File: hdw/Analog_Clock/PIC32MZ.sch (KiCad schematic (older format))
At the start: 3 parts

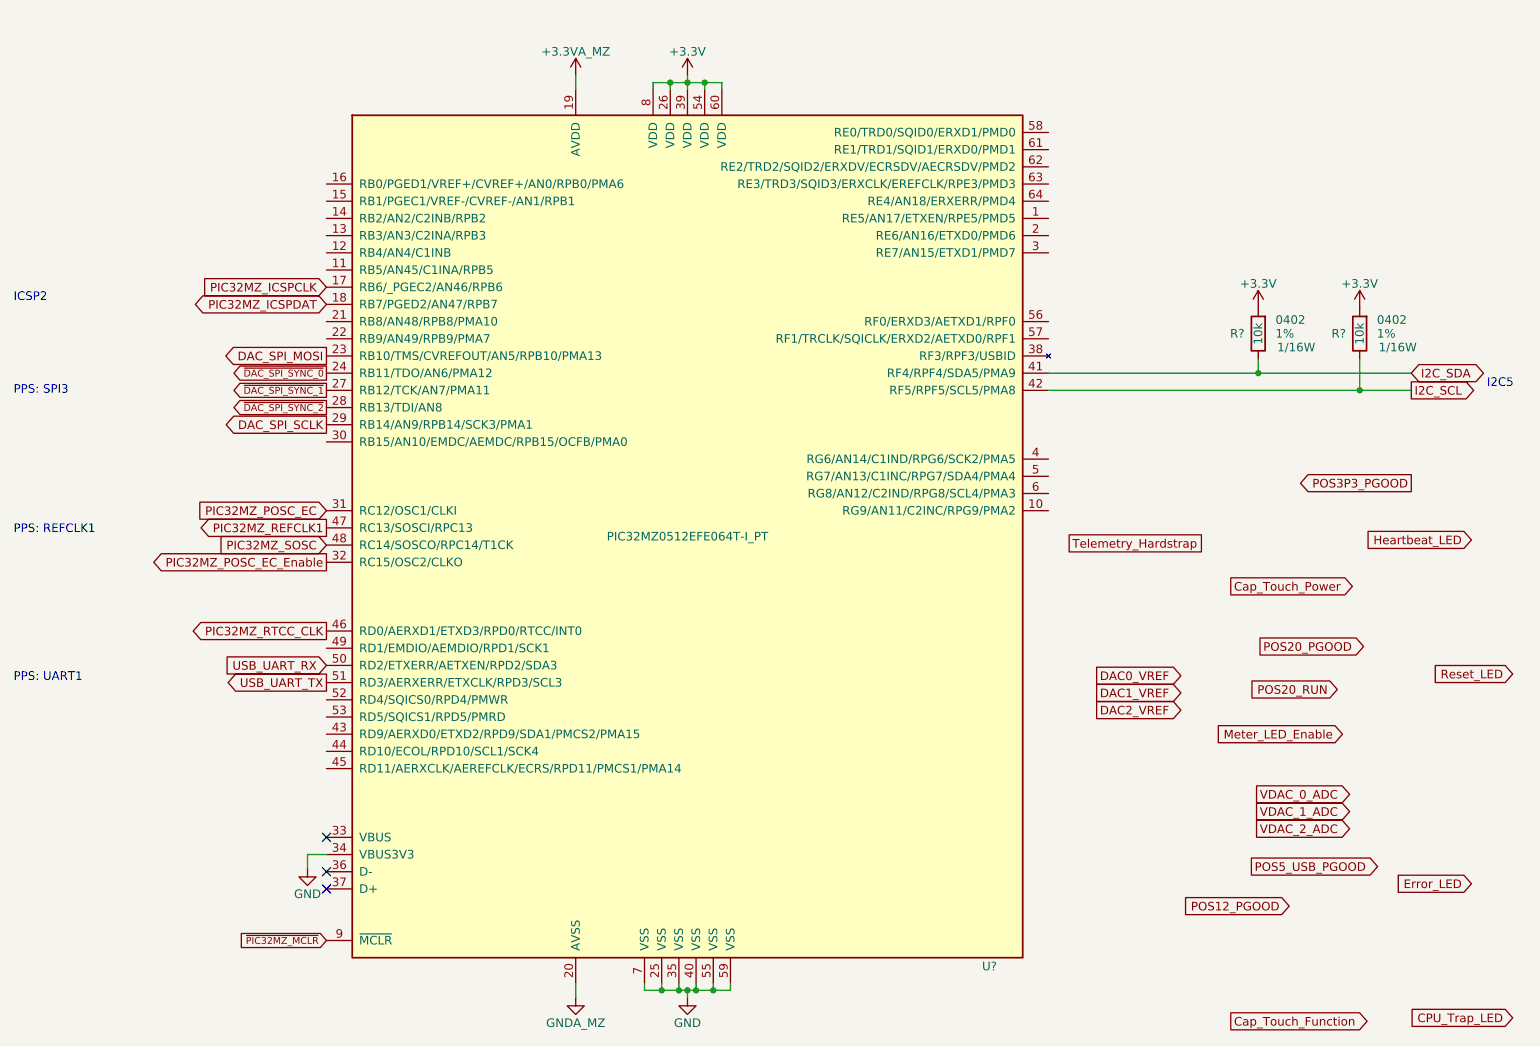
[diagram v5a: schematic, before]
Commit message: big sch push
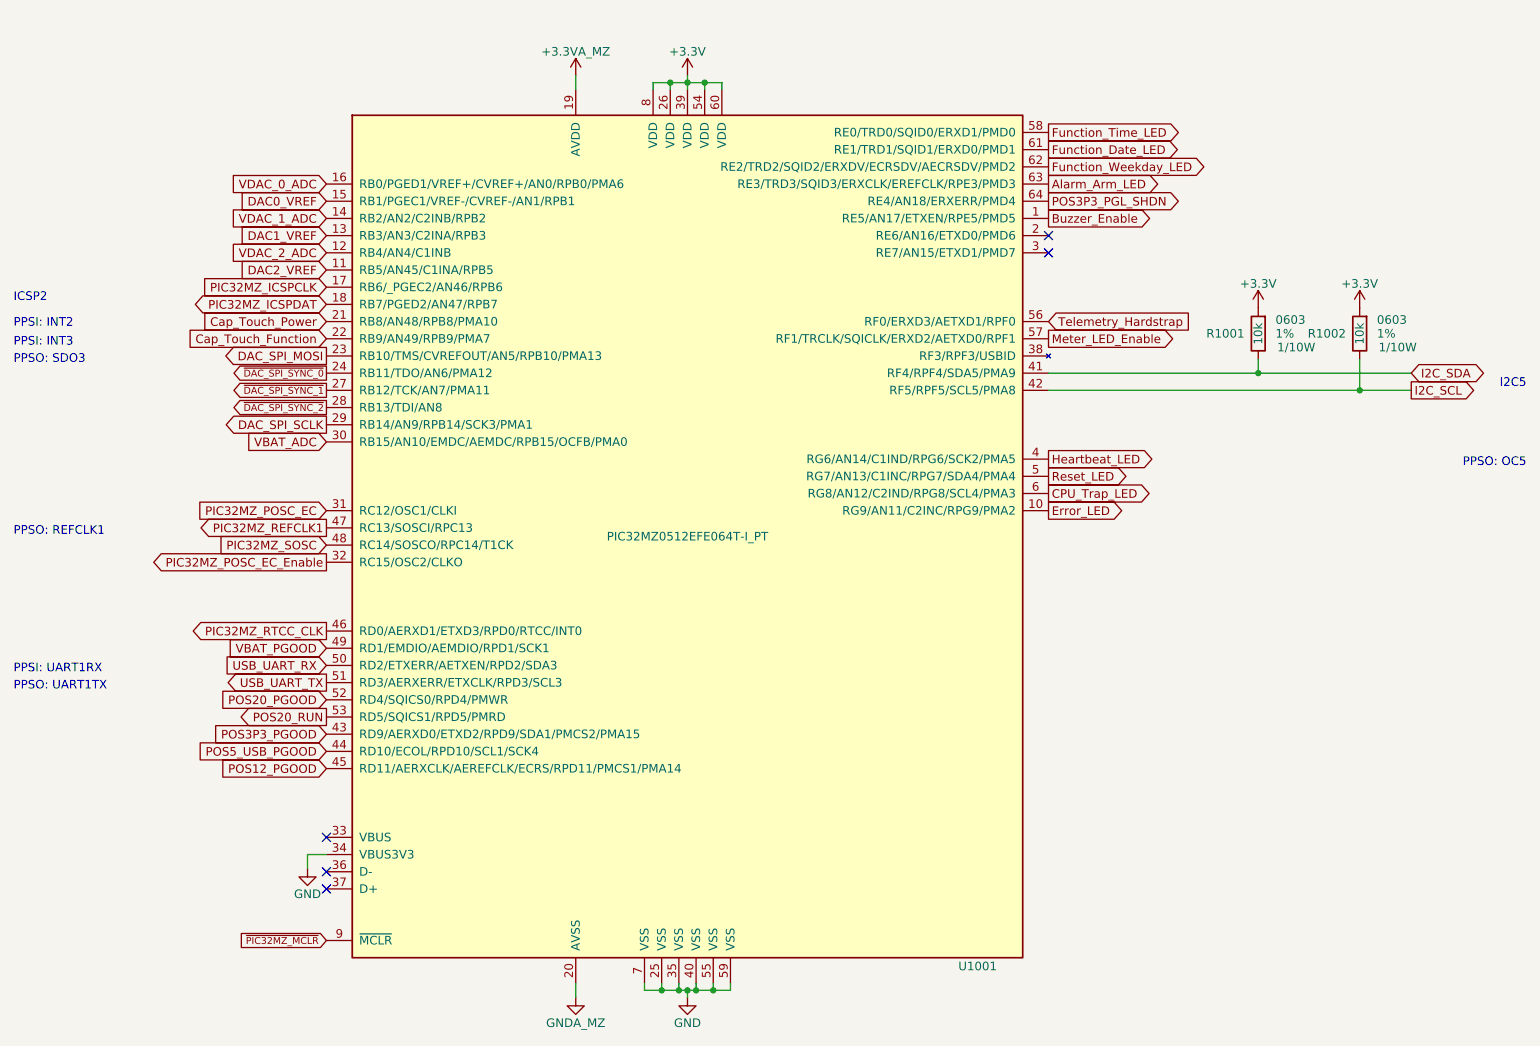
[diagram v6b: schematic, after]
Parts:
- R1001, R1002: renamed from R?; footprint Resistors_SMD:R_0402 -> Resistors_SMD:R_0603; Digi-Key PN RMCF0402FT10K0CT-ND -> (none); Wattage 1/16W -> 1/10W; display_footprint 0402 -> 0603
- gave numbers to parts that had none: 1
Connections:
- net CPU_Trap_LED: now also U1001.6 (RG8/AN12/C2IND/RPG8/SCL4/PMA3)
- net Cap_Touch_Function: now also U1001.22 (RB9/AN49/RPB9/PMA7)
- net Cap_Touch_Power: now also U1001.21 (RB8/AN48/RPB8/PMA10)
- net DAC0_VREF: now also U1001.15 (RB1/PGEC1/VREF-/CVREF-/AN1/RPB1)
- net DAC1_VREF: now also U1001.13 (RB3/AN3/C2INA/RPB3)
- net DAC2_VREF: now also U1001.11 (RB5/AN45/C1INA/RPB5)
- net Error_LED: now also U1001.10 (RG9/AN11/C2INC/RPG9/PMA2)
- net Heartbeat_LED: now also U1001.4 (RG6/AN14/C1IND/RPG6/SCK2/PMA5)
- net Meter_LED_Enable: now also U1001.57 (RF1/TRCLK/SQICLK/ERXD2/AETXD0/RPF1)
- net POS12_PGOOD: now also U1001.45 (RD11/AERXCLK/AEREFCLK/ECRS/RPD11/PMCS1/PMA14)
- net POS20_PGOOD: now also U1001.52 (RD4/SQICS0/RPD4/PMWR)
- net POS20_RUN: now also U1001.53 (RD5/SQICS1/RPD5/PMRD)
- net POS3P3_PGOOD: now also U1001.43 (RD9/AERXD0/ETXD2/RPD9/SDA1/PMCS2/PMA15)
- net POS5_USB_PGOOD: now also U1001.44 (RD10/ECOL/RPD10/SCL1/SCK4)
- net Reset_LED: now also U1001.5 (RG7/AN13/C1INC/RPG7/SDA4/PMA4)
- net Telemetry_Hardstrap: now also U1001.56 (RF0/ERXD3/AETXD1/RPF0)
- net VDAC_0_ADC: now also U1001.16 (RB0/PGED1/VREF+/CVREF+/AN0/RPB0/PMA6)
- net VDAC_1_ADC: now also U1001.14 (RB2/AN2/C2INB/RPB2)
- net VDAC_2_ADC: now also U1001.12 (RB4/AN4/C1INB)
- net Buzzer_Enable: now reaches U1001.1 (RE5/AN17/ETXEN/RPE5/PMD5)
- net VBAT_ADC: now reaches U1001.30 (RB15/AN10/EMDC/AEMDC/RPB15/OCFB/PMA0)
- net VBAT_PGOOD: now reaches U1001.49 (RD1/EMDIO/AEMDIO/RPD1/SCK1)
- net Function_Time_LED: now reaches U1001.58 (RE0/TRD0/SQID0/ERXD1/PMD0)
- net Function_Date_LED: now reaches U1001.61 (RE1/TRD1/SQID1/ERXD0/PMD1)
- net Function_Weekday_LED: now reaches U1001.62 (RE2/TRD2/SQID2/ERXDV/ECRSDV/AECRSDV/PMD2)
- net Alarm_Arm_LED: now reaches U1001.63 (RE3/TRD3/SQID3/ERXCLK/EREFCLK/RPE3/PMD3)
- net POS3P3_PGL_SHDN: now reaches U1001.64 (RE4/AN18/ERXERR/PMD4)
- no-connect marks 3 -> 5
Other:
- note added: "PPSI: INT2"
- note added: "PPSI: INT3"
- note added: "PPSI: UART1RX"
- note added: "PPSO: OC5"
- note added: "PPSO: REFCLK1"
- note added: "PPSO: SDO3"
- note added: "PPSO: UART1TX"
- note removed: "PPS: REFCLK1"
- note removed: "PPS: SPI3"
- note removed: "PPS: UART1"
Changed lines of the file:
@@
 $Descr A 11000 8500
 encoding utf-8
-Sheet 10 24
+Sheet 10 25
 Title "Pulse Oximeter"
 Date "2020-08-01"
@@
 	5620 1090 5520 1090
 $Comp
-L power:GND #PWR?
+L power:GND #PWR01005
 U 1 1 5CB03EF2
 P 5420 6410
-F 0 "#PWR?" H 5420 6160 50  0001 C CNN
+F 0 "#PWR01005" H 5420 6160 50  0001 C CNN
 F 1 "GND" H 5420 6260 50  0000 C CNN
 F 2 "" H 5420 6410 50  0001 C CNN
@@
 ~PIC32MZ_MCLR
 $Comp
-L power:GND #PWR?
+L power:GND #PWR01001
 U 1 1 5CB14B21
 P 3210 5660
-F 0 "#PWR?" H 3210 5410 50  0001 C CNN
+F 0 "#PWR01001" H 3210 5410 50  0001 C CNN
 F 1 "GND" H 3210 5510 50  0000 C CNN
 F 2 "" H 3210 5660 50  0001 C CNN
@@
 USB_UART_TX
 $Comp
-L power:+3.3V #PWR?
+L power:+3.3V #PWR01004
 U 1 1 5E6E7B25
 P 5420 1050
-F 0 "#PWR?" H 5420 900 50  0001 C CNN
+F 0 "#PWR01004" H 5420 900 50  0001 C CNN
 F 1 "+3.3V" H 5420 1190 50  0000 C CNN
 F 2 "" H 5420 1050 50  0001 C CNN
@@
 $EndComp
 $Comp
-L Custom_Library:+3.3VA_MZ #PWR?
+L Custom_Library:+3.3VA_MZ #PWR01002
 U 1 1 5EB1FED1
 P 4770 1050
-F 0 "#PWR?" H 4770 900 50  0001 C CNN
+F 0 "#PWR01002" H 4770 900 50  0001 C CNN
 F 1 "+3.3VA_MZ" H 4770 1190 50  0000 C CNN
 F 2 "" H 4770 1050 50  0001 C CNN
@@
 $EndComp
 $Comp
-L Custom_Library:GNDA_MZ #PWR?
+L Custom_Library:GNDA_MZ #PWR01003
 U 1 1 5EB20397
 P 4770 6410
-F 0 "#PWR?" H 4770 6160 50  0001 C CNN
+F 0 "#PWR01003" H 4770 6160 50  0001 C CNN
 F 1 "GNDA_MZ" H 4770 6260 50  0000 C CNN
 F 2 "" H 4770 6410 50  0001 C CNN
@@
 AR Path="/5EAE4A89/5EB7DAD1" Ref="R?"  Part="1"
 AR Path="/5EAE2F23/5EB7DAD1" Ref="R?"  Part="1"
-AR Path="/5E939ED2/5EB7DAD1" Ref="R?"  Part="1"
-F 0 "R?" H 9250 2550 50  0000 R CNN
+AR Path="/5E939ED2/5EB7DAD1" Ref="R1002"  Part="1"
+F 0 "R1002" H 9250 2550 50  0000 R CNN
 F 1 "10k" V 9330 2550 50  0000 C CNN
-F 2 "Resistors_SMD:R_0402" H 9330 2550 50  0001 C CNN
+F 2 "Resistors_SMD:R_0603" H 9330 2550 50  0001 C CNN
 F 3 "" H 9330 2550 50  0001 C CNN
-F 4 "0402" H 9430 2630 50  0000 L CNN "display_footprint"
+F 4 "0603" H 9430 2630 50  0000 L CNN "display_footprint"
 F 5 "1%" H 9430 2550 50  0000 L CNN "Tolerance"
-F 6 "1/16W" H 9440 2470 50  0000 L CNN "Wattage"
-F 7 "RMCF0402FT10K0CT-ND" H 9330 2550 50  0001 C CNN "Digi-Key PN"
+F 6 "1/10W" H 9440 2470 50  0000 L CNN "Wattage"
+F 7 "" H 9330 2550 50  0001 C CNN "Digi-Key PN"
 	1    9330 2550
 	1    0    0    -1
 $EndComp
 $Comp
-L power:+3.3V #PWR?
+L power:+3.3V #PWR01007
 U 1 1 5EB7DAD7
 P 9330 2400
-F 0 "#PWR?" H 9330 2250 50  0001 C CNN
+F 0 "#PWR01007" H 9330 2250 50  0001 C CNN
 F 1 "+3.3V" H 9330 2540 50  0000 C CNN
 F 2 "" H 9330 2400 50  0001 C CNN
@@
 AR Path="/5EAE4A89/5EB7DEAB" Ref="R?"  Part="1"
 AR Path="/5EAE2F23/5EB7DEAB" Ref="R?"  Part="1"
-AR Path="/5E939ED2/5EB7DEAB" Ref="R?"  Part="1"
-F 0 "R?" H 8660 2550 50  0000 R CNN
+AR Path="/5E939ED2/5EB7DEAB" Ref="R1001"  Part="1"
+F 0 "R1001" H 8660 2550 50  0000 R CNN
 F 1 "10k" V 8740 2550 50  0000 C CNN
-F 2 "Resistors_SMD:R_0402" H 8740 2550 50  0001 C CNN
+F 2 "Resistors_SMD:R_0603" H 8740 2550 50  0001 C CNN
 F 3 "" H 8740 2550 50  0001 C CNN
-F 4 "0402" H 8840 2630 50  0000 L CNN "display_footprint"
+F 4 "0603" H 8840 2630 50  0000 L CNN "display_footprint"
 F 5 "1%" H 8840 2550 50  0000 L CNN "Tolerance"
-F 6 "1/16W" H 8850 2470 50  0000 L CNN "Wattage"
-F 7 "RMCF0402FT10K0CT-ND" H 8740 2550 50  0001 C CNN "Digi-Key PN"
+F 6 "1/10W" H 8850 2470 50  0000 L CNN "Wattage"
+F 7 "" H 8740 2550 50  0001 C CNN "Digi-Key PN"
 	1    8740 2550
 	1    0    0    -1
 $EndComp
 $Comp
-L power:+3.3V #PWR?
+L power:+3.3V #PWR01006
 U 1 1 5EB7DEB5
 P 8740 2400
-F 0 "#PWR?" H 8740 2250 50  0001 C CNN
+F 0 "#PWR01006" H 8740 2250 50  0001 C CNN
 F 1 "+3.3V" H 8740 2540 50  0000 C CNN
 F 2 "" H 8740 2400 50  0001 C CNN
@@
 PIC32MZ_SOSC
 $Comp
-L Custom_Library:PIC32MZ0512EFE064T-I_PT U?
+L Custom_Library:PIC32MZ0512EFE064T-I_PT U1001
 U 1 1 5F3A240D
 P 5420 3730
-F 0 "U?" H 7220 1230 50  0000 R CNN
+F 0 "U1001" H 7220 1230 50  0000 R CNN
 F 1 "PIC32MZ0512EFE064T-I_PT" H 5420 3730 50  0000 C CNN
 F 2 "Package_QFP:TQFP-64_10x10mm_P0.5mm" H 5420 3730 50  0001 C CNN
@@
 	1    0    0    -1
 $EndComp
-Text Notes 10070 2870 0    50   ~ 0
+Text Notes 10300 2870 2    50   ~ 0
 I2C5
-Text Notes 1500 4580 0    50   ~ 0
-PPS: UART1
-Text Notes 1500 3720 0    50   ~ 0
-PPS: REFCLK1
+Text Notes 1500 4530 0    50   ~ 0
+PPSI: UART1RX
+Text Notes 1500 3730 0    50   ~ 0
+PPSO: REFCLK1
 Text GLabel 3320 2680 0    50   Output ~ 0
 DAC_SPI_MOSI
@@
 Text GLabel 3320 2980 0    40   Output ~ 0
 ~DAC_SPI_SYNC_2
-Text Notes 1500 2910 0    50   ~ 0
-PPS: SPI3
-Text GLabel 8730 5230 2    50   Output ~ 0
+Text Notes 1500 2730 0    50   ~ 0
+PPSO: SDO3
+Text GLabel 3320 1680 0    50   Input ~ 0
 VDAC_0_ADC
-Text GLabel 8730 5330 2    50   Output ~ 0
+Text GLabel 3320 1880 0    50   Input ~ 0
 VDAC_1_ADC
-Text GLabel 8730 5430 2    50   Output ~ 0
+Text GLabel 3320 2080 0    50   Input ~ 0
 VDAC_2_ADC
 Text Notes 1500 2370 0    50   ~ 0
@@
 Text GLabel 3320 4280 0    50   Output ~ 0
 PIC32MZ_RTCC_CLK
-Text GLabel 9230 4880 0    50   Input ~ 0
+Text GLabel 7520 2580 2    50   Output ~ 0
 Meter_LED_Enable
-Text GLabel 8580 4020 2    50   Output ~ 0
+Text GLabel 3320 2480 0    50   Input ~ 0
 Cap_Touch_Power
-Text GLabel 8580 6550 2    50   Output ~ 0
+Text GLabel 3320 2580 0    50   Input ~ 0
 Cap_Touch_Function
-Text GLabel 9200 4620 0    50   Input ~ 0
+Text GLabel 3320 4780 0    50   Output ~ 0
 POS20_RUN
-Text GLabel 8750 4370 2    50   Output ~ 0
+Text GLabel 3320 4680 0    50   Input ~ 0
 POS20_PGOOD
-Text GLabel 8920 5880 0    50   Input ~ 0
+Text GLabel 3320 5080 0    50   Input ~ 0
 POS12_PGOOD
-Text GLabel 9630 3420 0    50   Output ~ 0
+Text GLabel 3320 4880 0    50   Input ~ 0
 POS3P3_PGOOD
-Text GLabel 8700 5650 2    50   Output ~ 0
+Text GLabel 3320 4980 0    50   Input ~ 0
 POS5_USB_PGOOD
-Text GLabel 9980 3750 0    50   Input ~ 0
+Text GLabel 7520 3280 2    50   Output ~ 0
 Heartbeat_LED
-Text GLabel 9980 5750 0    50   Input ~ 0
+Text GLabel 7520 3580 2    50   Output ~ 0
 Error_LED
-Text GLabel 10220 4530 0    50   Input ~ 0
+Text GLabel 7520 3380 2    50   Output ~ 0
 Reset_LED
-Text GLabel 10220 6530 0    50   Input ~ 0
+Text GLabel 3320 1780 0    50   Input ~ 0
+DAC0_VREF
+Text GLabel 3320 1980 0    50   Input ~ 0
+DAC1_VREF
+Text GLabel 3320 2180 0    50   Input ~ 0
+DAC2_VREF
+Text GLabel 7520 2480 2    50   Input ~ 0
+Telemetry_Hardstrap
+Text GLabel 3320 3180 0    50   Input ~ 0
+VBAT_ADC
+Text Notes 1500 2520 0    50   ~ 0
+PPSI: INT2
+Text Notes 1500 2630 0    50   ~ 0
+PPSI: INT3
+Text Notes 1500 4630 0    50   ~ 0
+PPSO: UART1TX
+Text Notes 10300 3330 2    50   ~ 0
+PPSO: OC5
+Text GLabel 7520 3480 2    50   Output ~ 0
 CPU_Trap_LED
-Text GLabel 7800 4540 2    50   Output ~ 0
-DAC0_VREF
-Text GLabel 7800 4640 2    50   Output ~ 0
-DAC1_VREF
-Text GLabel 7800 4740 2    50   Output ~ 0
-DAC2_VREF
-Text GLabel 7640 3770 2    50   UnSpc ~ 0
-Telemetry_Hardstrap
+Text GLabel 3320 4380 0    50   Input ~ 0
+VBAT_PGOOD
+Text GLabel 7520 1480 2    50   Output ~ 0
+Function_Date_LED
+Text GLabel 7520 1380 2    50   Output ~ 0
+Function_Time_LED
+Text GLabel 7520 1580 2    50   Output ~ 0
+Function_Weekday_LED
+Text GLabel 7520 1680 2    50   Output ~ 0
+Alarm_Arm_LED
+NoConn ~ 7520 1980
+NoConn ~ 7520 2080
+Text GLabel 7520 1780 2    50   Output ~ 0
+POS3P3_PGL_SHDN
+Text GLabel 7520 1880 2    50   Output ~ 0
+Buzzer_Enable
 $EndSCHEMATC
